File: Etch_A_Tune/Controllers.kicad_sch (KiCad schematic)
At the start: 29 parts

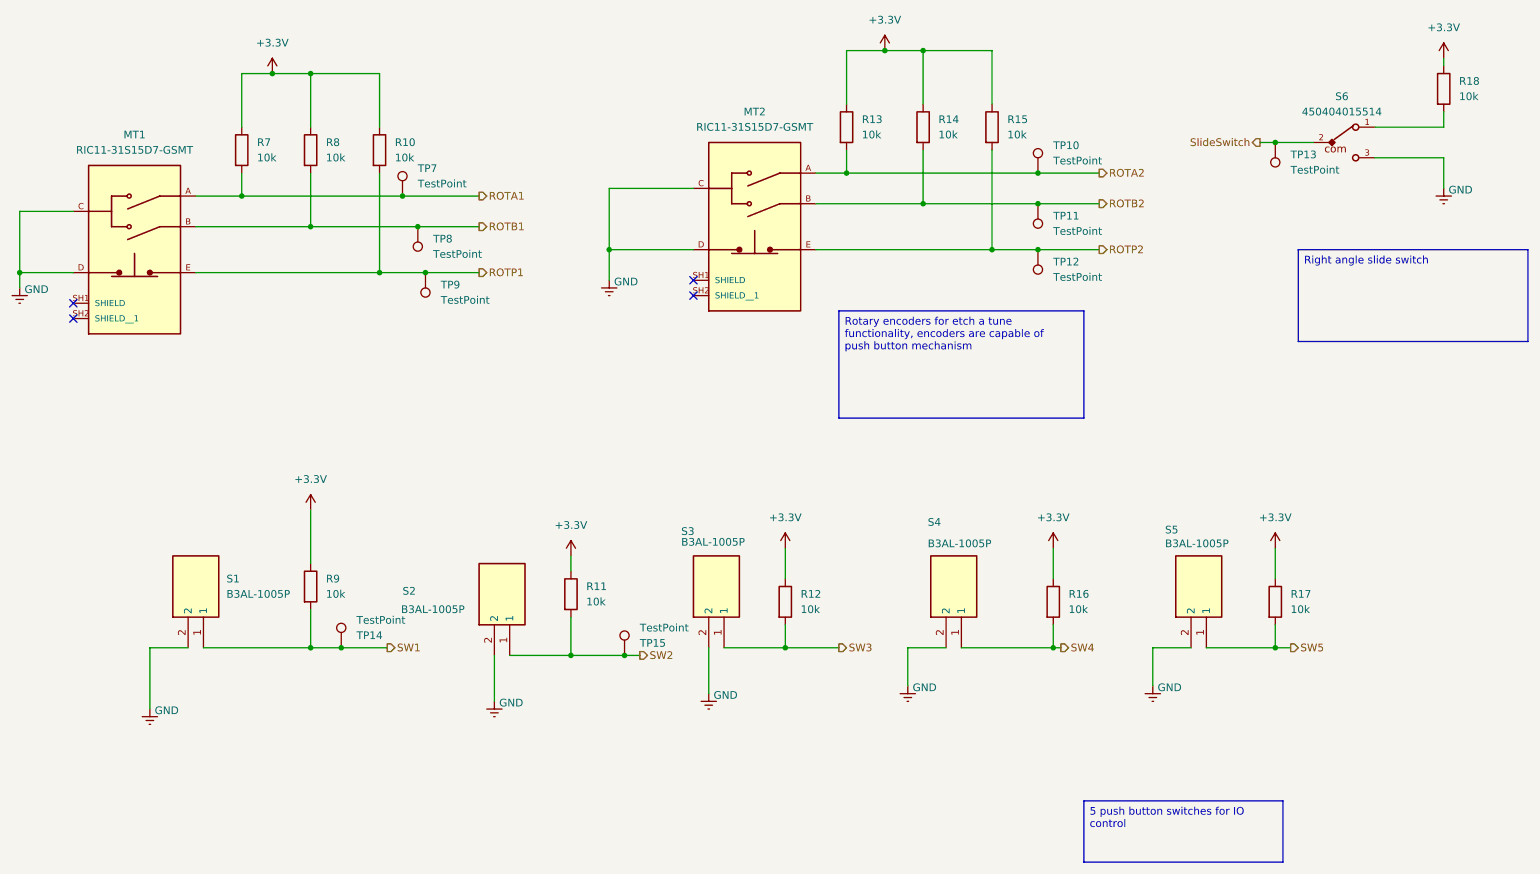
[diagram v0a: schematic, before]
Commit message: Another Update! :D
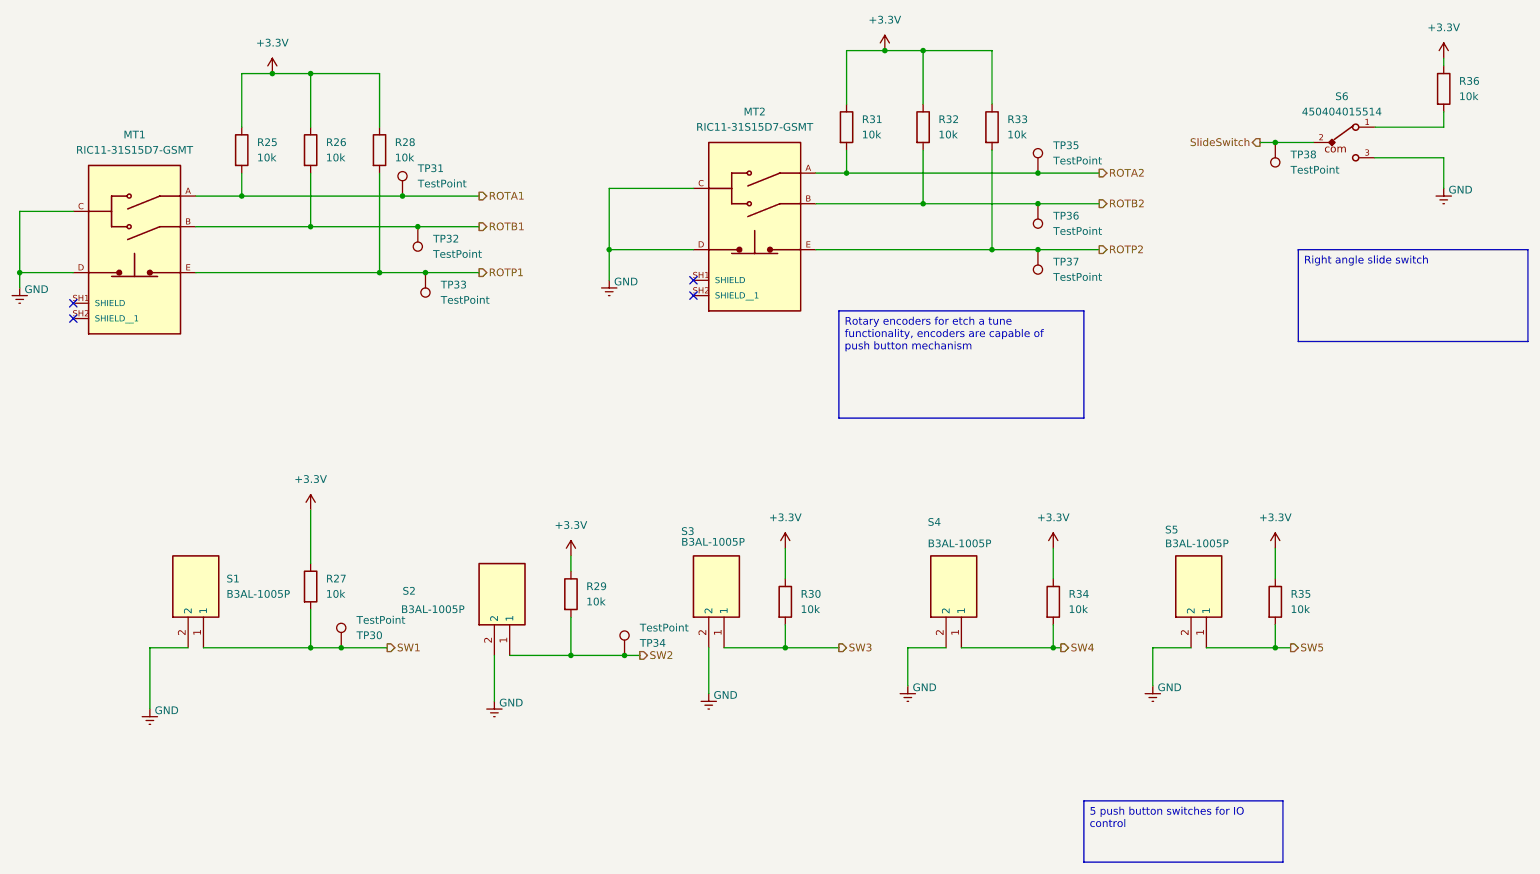
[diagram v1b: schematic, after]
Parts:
- renumbered R7 to R25, R8 to R26, R9 to R27, R10 to R28, R11 to R29, R12 to R30, R13 to R31, R14 to R32, R15 to R33, R16 to R34, R17 to R35, R18 to R36, TP14 to TP30, TP7 to TP31, TP8 to TP32, TP9 to TP33, TP15 to TP34, TP10 to TP35, TP11 to TP36, TP12 to TP37, TP13 to TP38

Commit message: pdf docs
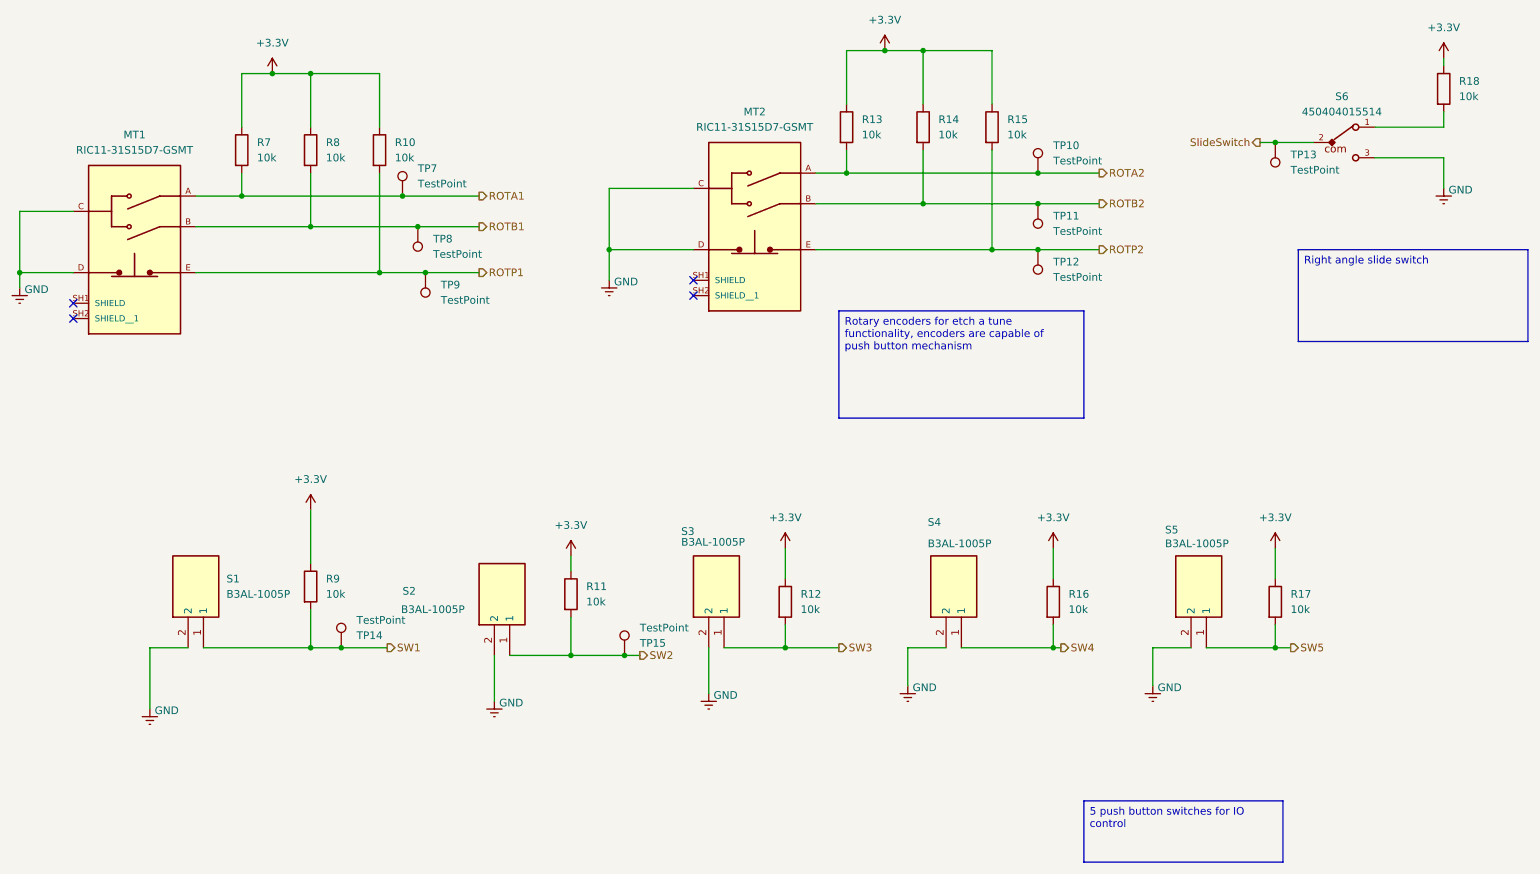
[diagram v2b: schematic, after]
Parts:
- renumbered R28 to R10, R29 to R11, R30 to R12, R31 to R13, R32 to R14, R33 to R15, R34 to R16, R35 to R17, R36 to R18, R25 to R7, R26 to R8, R27 to R9, TP35 to TP10, TP36 to TP11, TP37 to TP12, TP38 to TP13, TP30 to TP14, TP34 to TP15, TP31 to TP7, TP32 to TP8, TP33 to TP9
